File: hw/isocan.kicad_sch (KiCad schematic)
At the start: 16 parts, among them U10 ISO6521F, U12 TJA1051TK/3,118

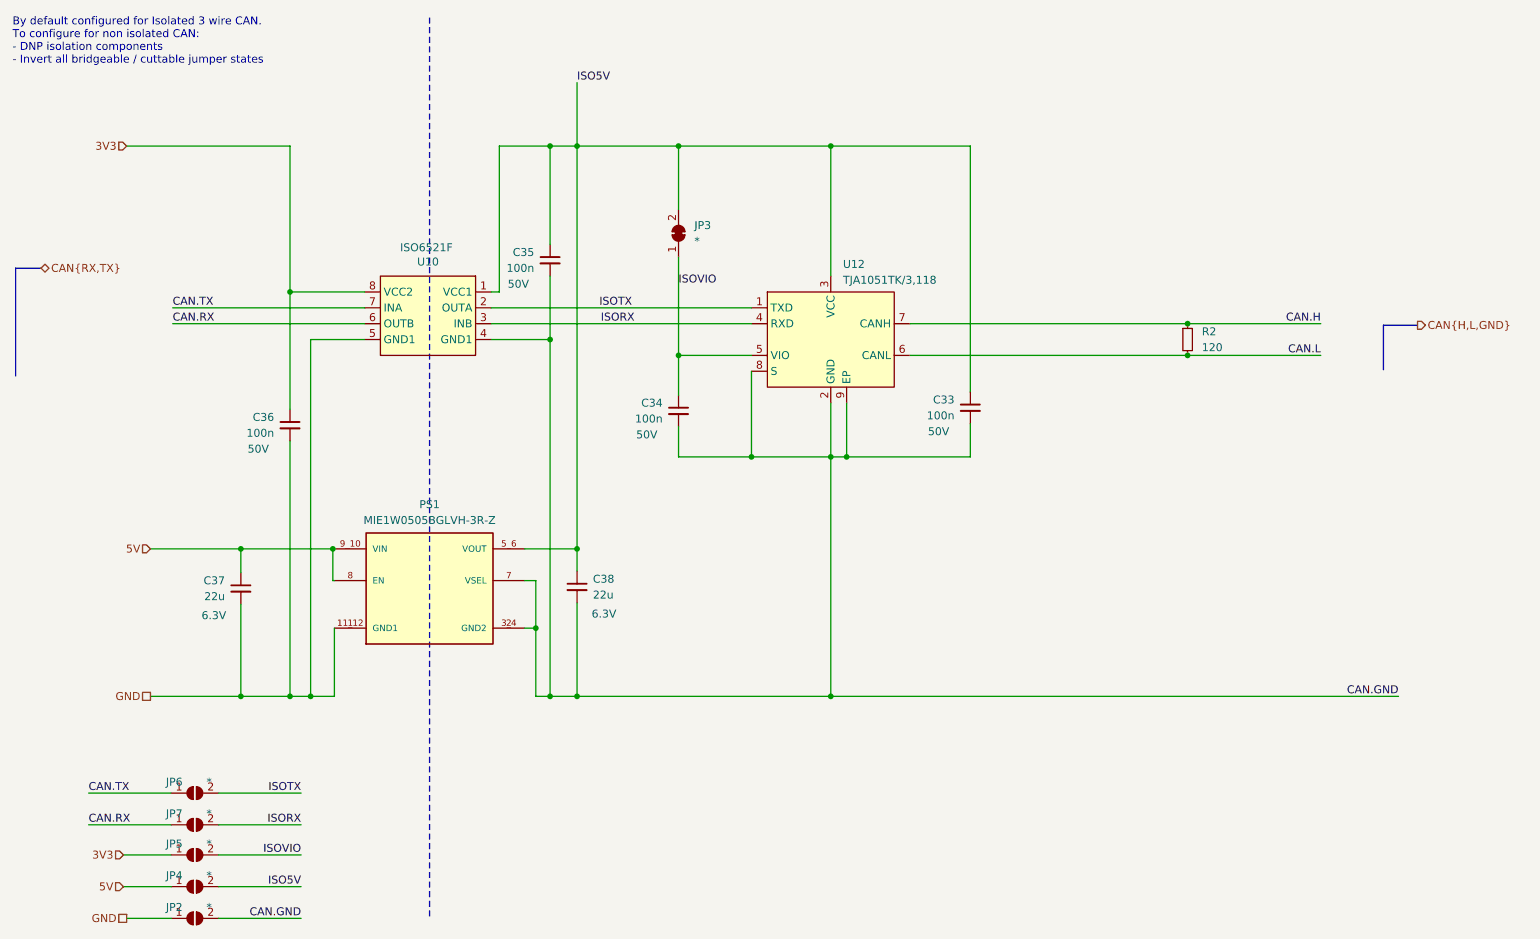
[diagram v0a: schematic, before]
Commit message: [Hw] WIP begun revisions for v0.2.0
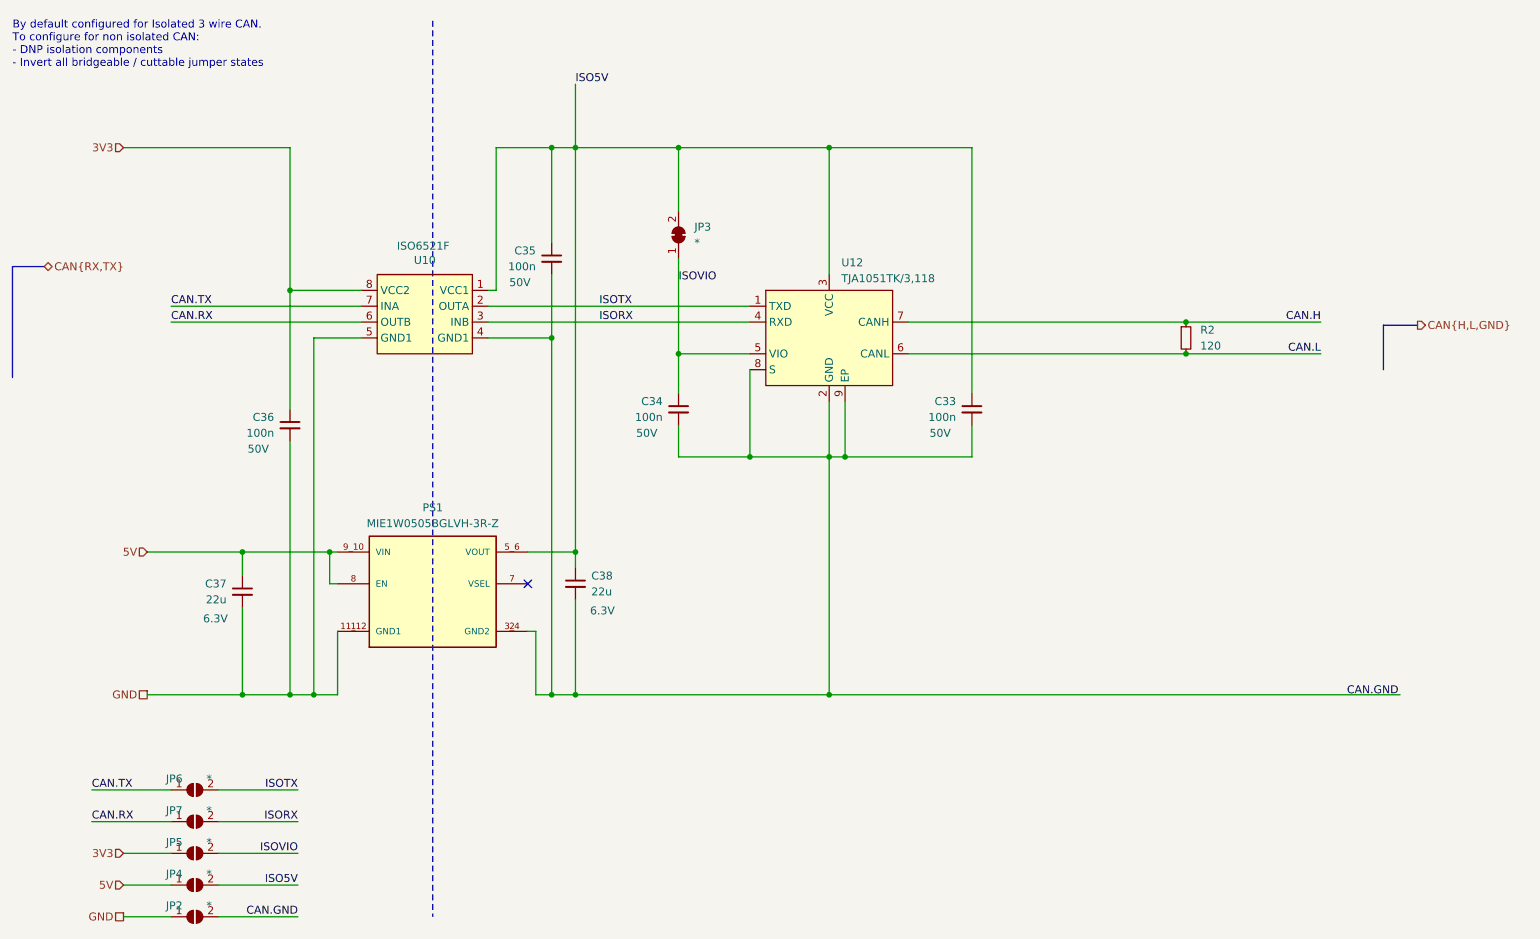
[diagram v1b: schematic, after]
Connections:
- net CAN.GND: no longer C33.2, C34.2, C35.2, C38.2, PS1.2 (GND2), PS1.3_4 (GND2), PS1.7 (VSEL), U10.4 (GND1), U12.2 (GND), U12.8 (S), U12.9 (EP)
- new net: C33.2, C34.2, C35.2, C38.2, PS1.2 (GND2), PS1.3_4 (GND2), U10.4 (GND1), U12.2 (GND), U12.8 (S), U12.9 (EP)
- no-connect marks 0 -> 1
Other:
- moved on the sheet: C37, C38, JP6, JP7, PS1, U10
